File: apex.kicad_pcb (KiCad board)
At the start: 4 copper layers, 65.4 x 30.5 mm, 57 parts, among them J1 Conn_01x04_Pin, J2 USB_C_Receptacle_USB2.0_16P, J3 Conn_01x04_Pin, J5 Conn_01x04_Pin, SW1 PCM12SMTR, SW2 KMR223G LFG, U1 AP7363-33D-13, U2 APX803L20-29SA-7, U4 STM32F070RBTx, U7 USBLC6-2P6, Y2 XRCGB32M000F2P01R0

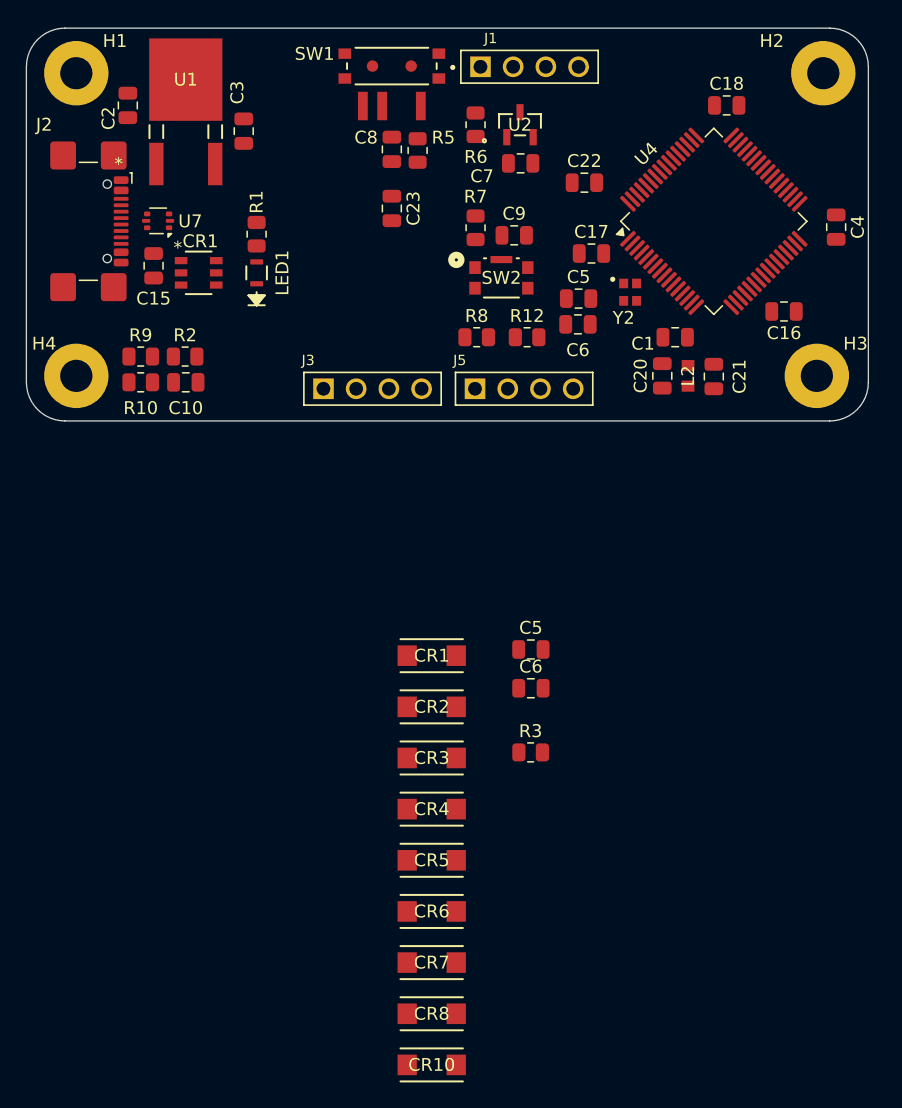
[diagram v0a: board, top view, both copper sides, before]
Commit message: added sheets
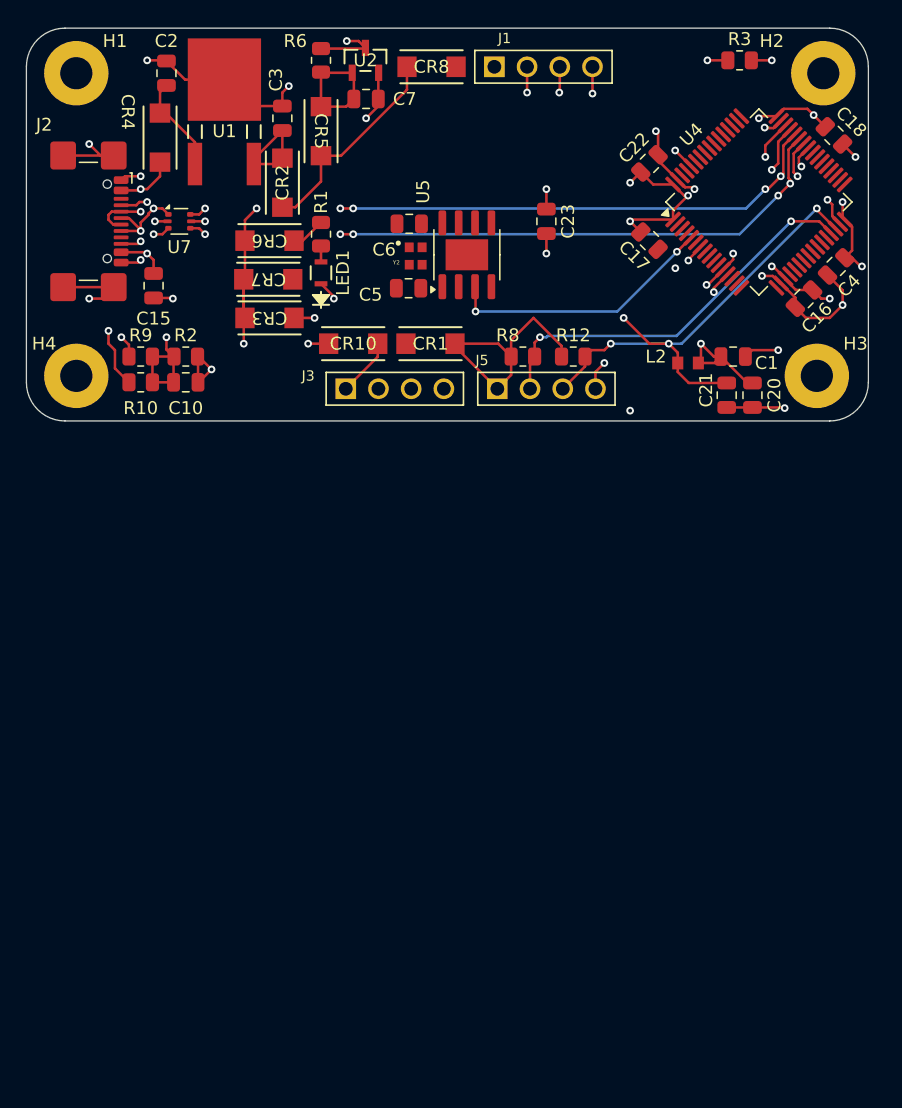
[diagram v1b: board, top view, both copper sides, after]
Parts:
- removed the C5 at (59.5, 52.0)
- removed the C6 at (59.5, 54.0)
- removed C8: 100 nF, Capacitor_SMD:C_0805_2012Metric
- removed C9: 47 nF, Capacitor_SMD:C_0805_2012Metric
- removed the CR1 at (30.0, 50.0)
- removed R5: 10K, Resistor_SMD:R_0805_2012Metric
- removed R7: 100K, Resistor_SMD:R_0805_2012Metric
- removed SW1: PCM12SMTR, PCM12SMTR:PCM12SMTR_CNK
- removed SW2: KMR223G LFG, KMR223_LFG:KMR2_G_CNK
- added U5: ~, Package_SO:SOIC-8-1EP_3.9x4.9mm_P1.27mm_EP2.41x3.3mm, F.Cu at (50.8, 48.6)
- J1: footprint PPTC041LFBN_RC:PPTC041LFBN-RC -> J_1x4:PPTC041LFBN-RC
- J3, J5: footprint PPTC041LFBN_RC:SULLINS_PPTC041LFBN-RC -> J_1x4:PPTC041LFBN-RC
- LED1: footprint 150080BS75000:150080BS75000 -> LED_0805_BLUE:150080BS75000
- Y2: footprint XRCGB32M000F2P01R0:OSC_XRCGB32M000F2P01R0 -> CRYSTAL_32MHZ:OSC_XRCGB32M000F2P01R0
- moved CR8 73.5 mm to (48.1, 34.0)
- moved CR5 57.3 mm to (39.5, 39.0), turned to -90 degrees
- moved CR10 56.3 mm to (42.0, 55.5)
- moved CR4 56.2 mm to (27.0, 39.5), turned to -90 degrees
- moved R3 56.1 mm to (72.0, 33.5)
- moved CR7 54.6 mm to (35.4, 50.5), turned to 180 degrees
- moved CR6 53.6 mm to (35.5, 47.5), turned to 180 degrees
- moved CR2 42.3 mm to (36.5, 43.0), turned to 90 degrees
- moved C6 37.3 mm to (46.4, 46.2)
- moved CR3 36.4 mm to (35.5, 53.5), turned to 180 degrees
- moved C5 29.6 mm to (46.3, 51.2)
- moved CR1 24.2 mm to (48.0, 55.5)
- moved Y2 16.9 mm to (46.9, 48.7)
- moved C7 13.0 mm to (43.0, 36.5)
- moved R6 13.0 mm to (39.5, 33.5)
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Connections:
- C5 pad 1: GND1 -> GND
- C6 pad 1: GND1 -> GND
- C7 pad 1: GND2 -> GND
- R3 pad 1: Net-(U4-BOOT0) -> Boot0
- U2 pad 2: GND2 -> GND
- U4 pad 60: Net-(U4-BOOT0) -> Boot0
- Y2 pad 1: HSE_IN -> XIN
- Y2 pad 3: HSE_OUT -> XOUT
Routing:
- net GND: track 0.00 -> 266.1 mm, vias 0 -> 26
- net VDD: track 0.00 -> 109.5 mm, vias 0 -> 13
- net USB_N: track 0.00 -> 52.7 mm, vias 0 -> 5
- net USB_P: track 0.00 -> 51.3 mm, vias 0 -> 5
- net GNDPWR: track 0.00 -> 42.4 mm, vias 0 -> 3
- net RST_L: track 0.00 -> 41.3 mm, vias 0 -> 2
- net VDC: track 0.00 -> 39.0 mm, vias 0 -> 3
- net +3V3: track 0.00 -> 32.8 mm
- net I2C2_SCL: track 0.00 -> 31.0 mm, vias 0 -> 2
- net I2C2_SDA: track 0.00 -> 28.2 mm, vias 0 -> 2
- net CLK_32MHZ: track 0.00 -> 20.5 mm, vias 0 -> 2
- net USB_CC1: track 0.00 -> 19.0 mm, vias 0 -> 2
- net VBUS: track 0.00 -> 15.5 mm, vias 0 -> 3
- net +3.3VA: track 0.00 -> 15.1 mm, vias 0 -> 2
- net USB_CC2: track 0.00 -> 11.4 mm, vias 0 -> 2
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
